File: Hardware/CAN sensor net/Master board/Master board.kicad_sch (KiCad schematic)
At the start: 45 parts, among them SW1 SW_Push, SW2 SW_SPDT, U1 STM32F405RGTx, U5 SN65HVD230, U6 SN65HVD230, U7 W25Q32FVSSIG, Y1 16MHz

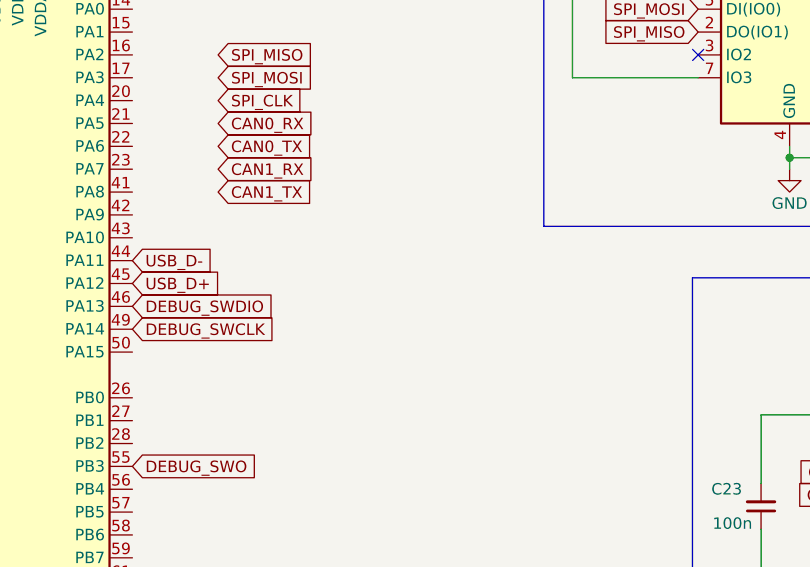
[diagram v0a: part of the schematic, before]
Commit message: added band pass filter to piezo board
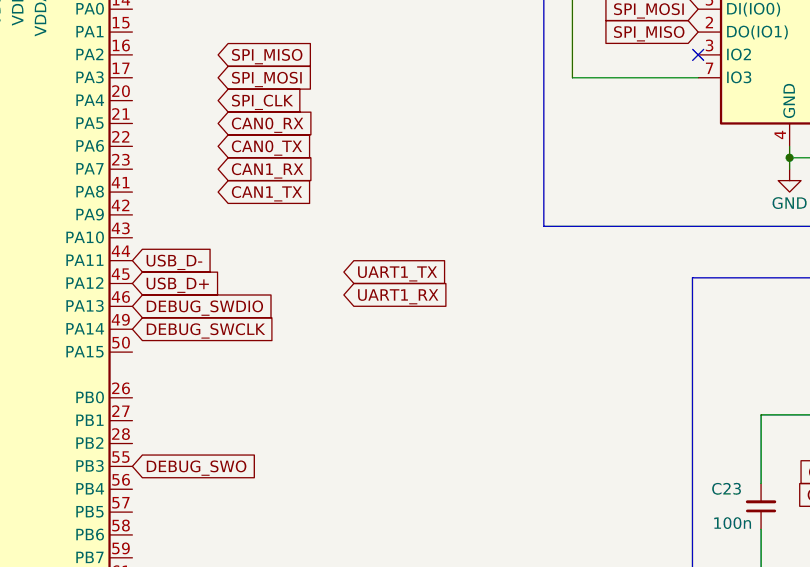
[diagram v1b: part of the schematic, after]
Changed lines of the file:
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@@
+		)
+	)
+	(global_label "UART1_TX"
+		(shape input)
+		(at 110.49 110.49 0)
+		(fields_autoplaced yes)
+		(effects
+			(font
+				(size 1.27 1.27)
+			)
+			(justify left)
+		)
+		(property "Intersheetrefs" "${INTERSHEET_REFS}"
+			(at 122.4861 110.49 0)
+			(effects
+				(font
+					(size 1.27 1.27)
+				)
+				(justify left)
+				(hide yes)
+			)
 		)
 	)
@@
 				(hide yes)
 			)
+		)
+	)
+	(global_label "UART1_RX"
+		(shape input)
+		(at 110.49 113.03 0)
+		(fields_autoplaced yes)
+		(effects
+			(font
+				(size 1.27 1.27)
+			)
+			(justify left)
+		)
+		(property "Intersheetrefs" "${INTERSHEET_REFS}"
+			(at 122.7885 113.03 0)
+			(effects
+				(font
+					(size 1.27 1.27)
+				)
+				(justify left)
+				(hide yes)
+			)
